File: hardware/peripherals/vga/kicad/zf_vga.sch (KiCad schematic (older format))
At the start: 3 parts

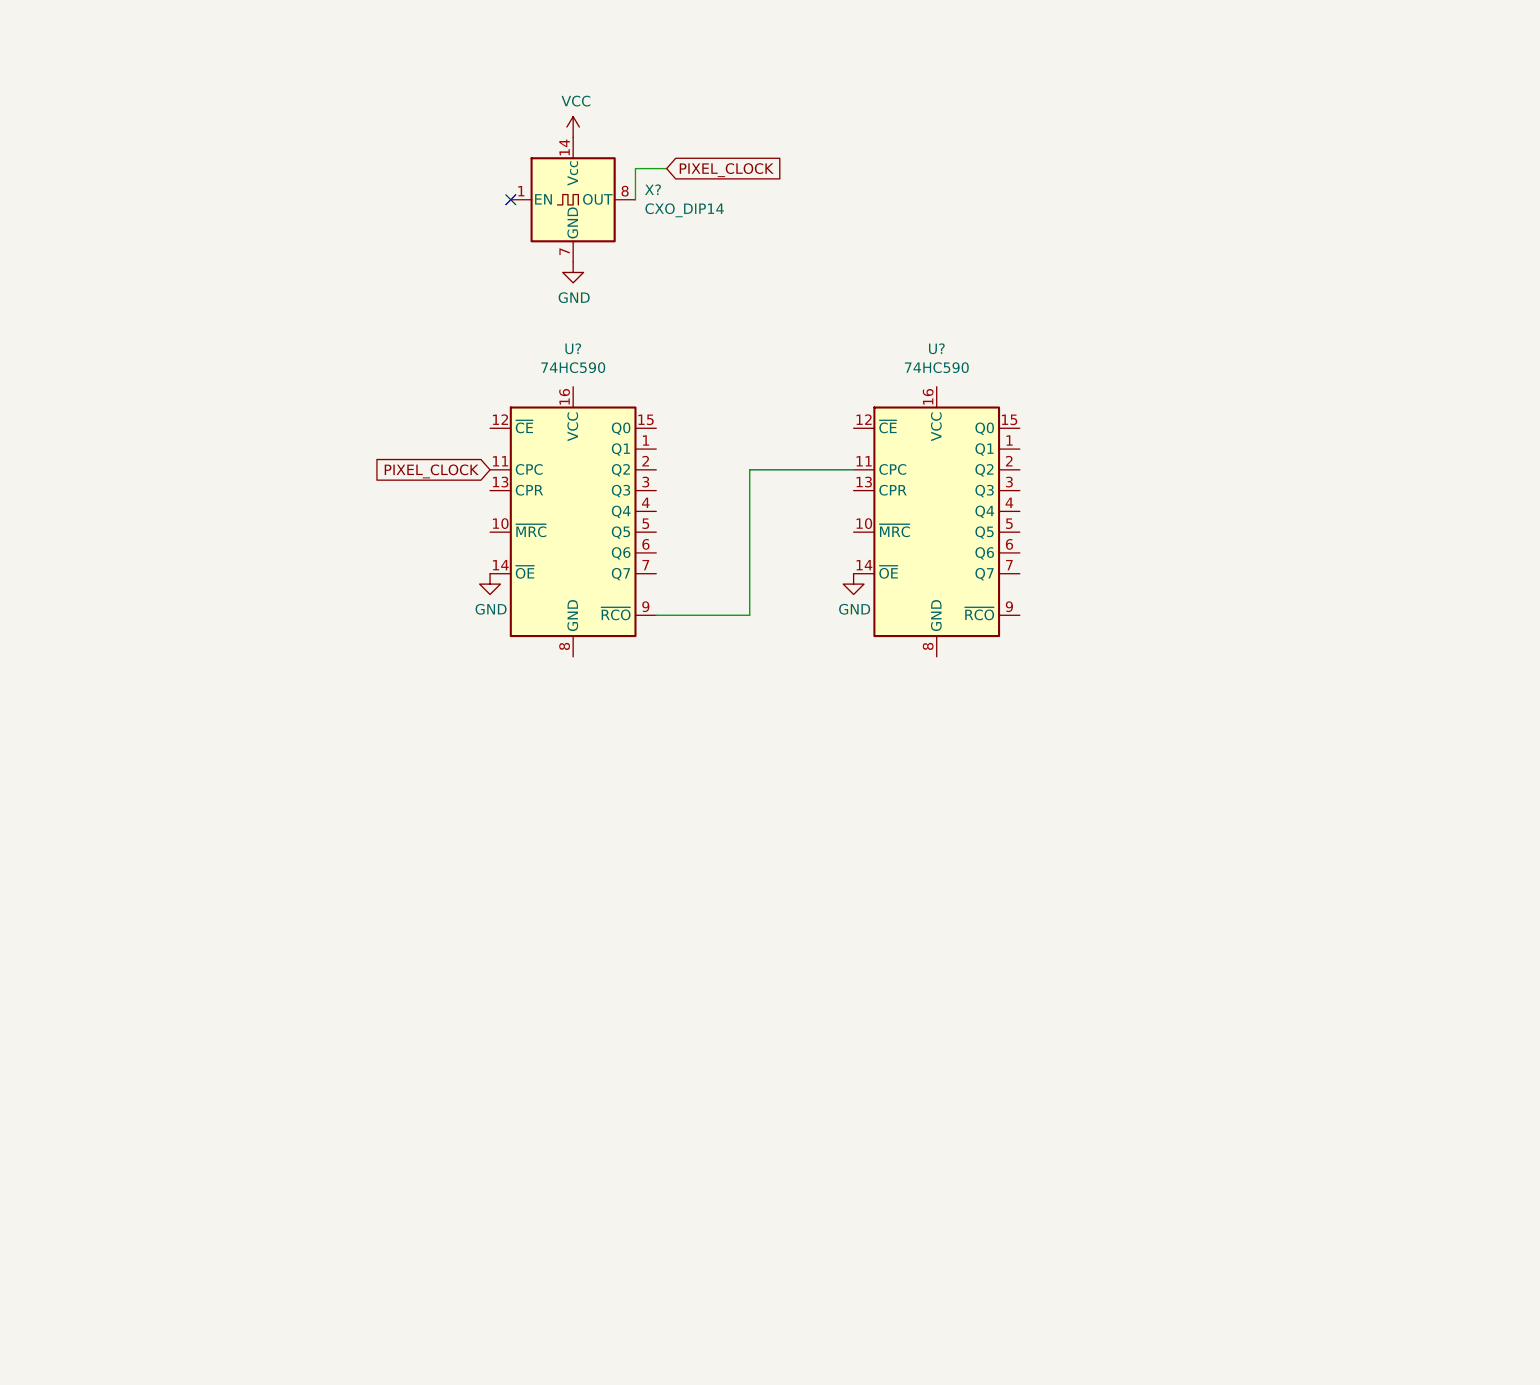
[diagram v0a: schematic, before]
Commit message: Generate test pattern
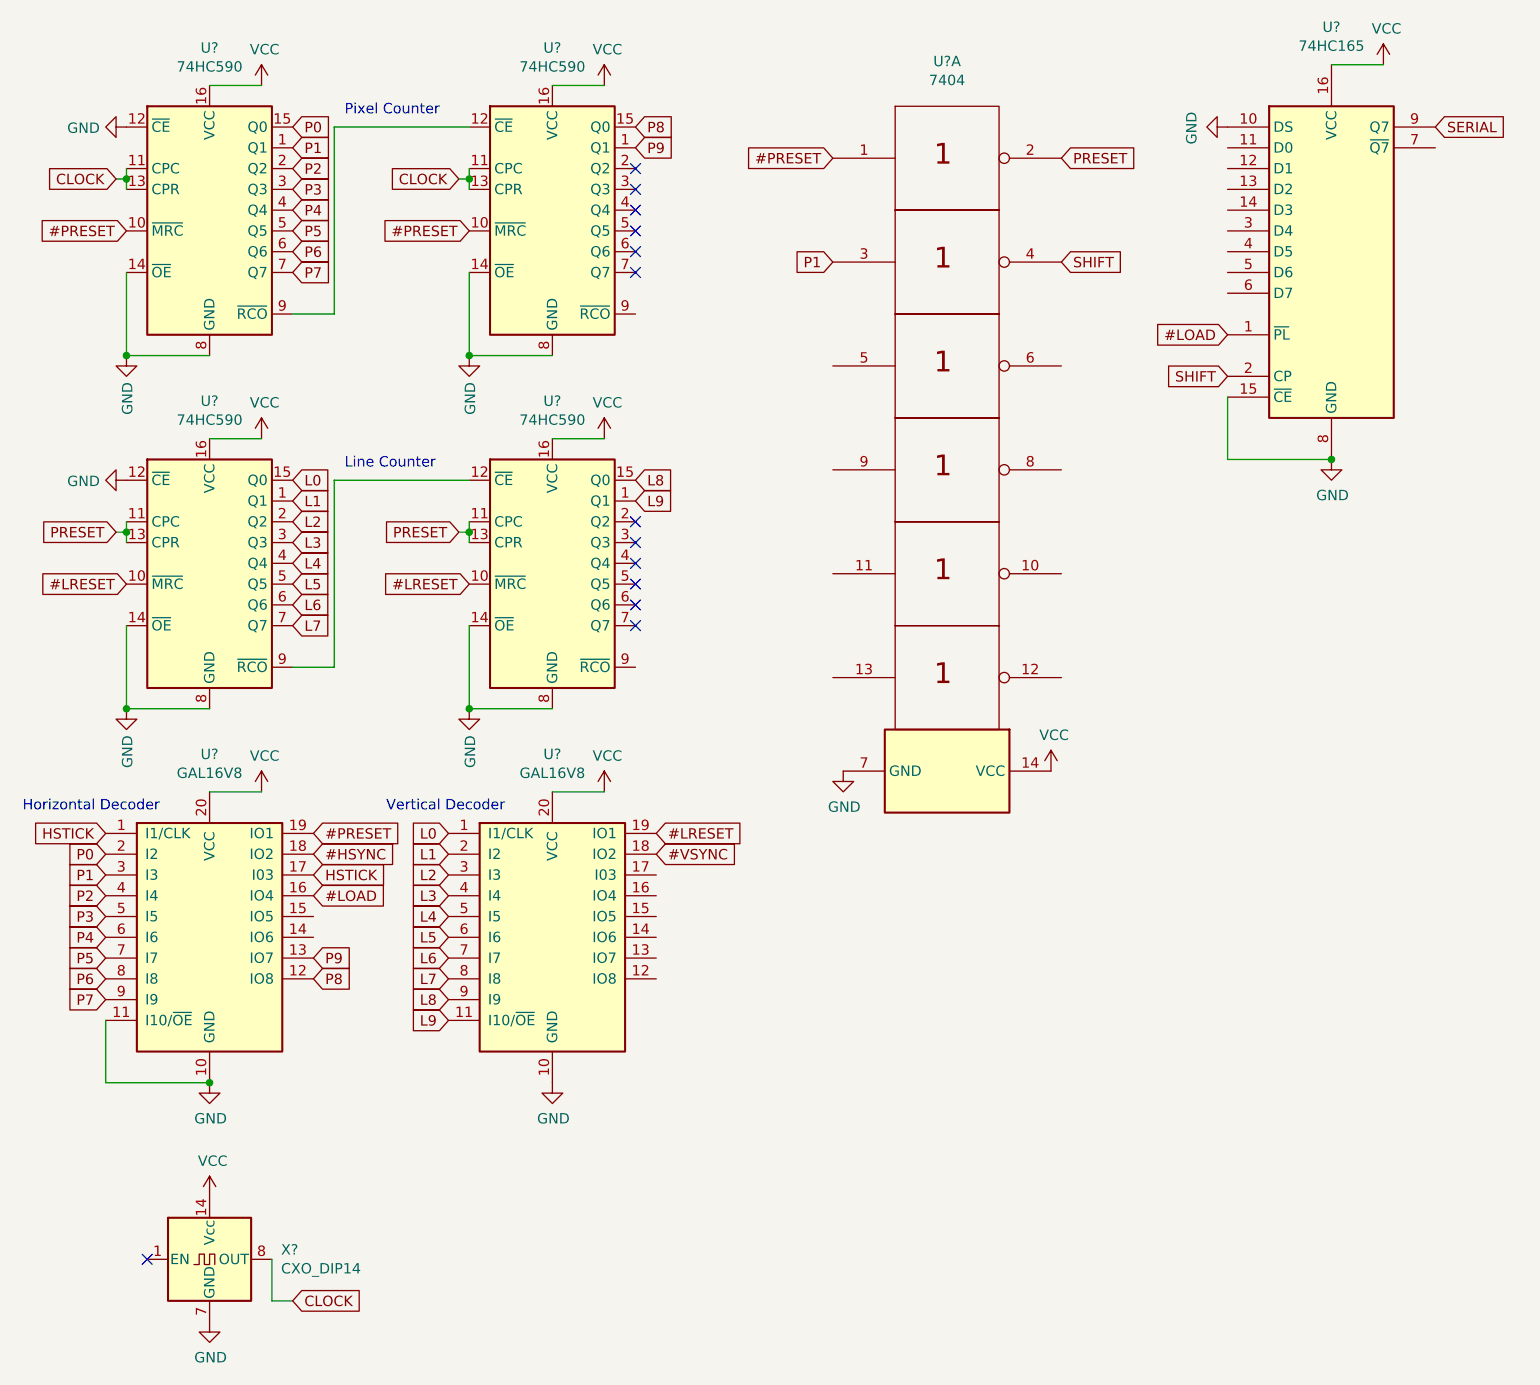
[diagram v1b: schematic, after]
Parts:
- removed U? (x2): 74HC590, symbol 74xx:74HC590
- added U? (x2): GAL16V8, symbol Logic_Programmable:GAL16V8
- added U? (x4): 74HC590, symbol 74xx:74HC590
- added U? (x6): 7404, symbol 74xx_IEEE:7404
- added U?: 74HC04, symbol 74xx:74HC04
- added U?: 74HC165, symbol 74xx:74HC165
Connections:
- net GND: now also U?.10 (DS), U?.10 (GND), U?.10 (GND), U?.11 (I10/~OE~), U?.12 (~CE), U?.12 (~CE), U?.14 (~OE), U?.14 (~OE), U?.14 (~OE), U?.14 (~OE), U?.15 (~CE), U?.7 (GND), U?.8 (GND), U?.8 (GND), U?.8 (GND), U?.8 (GND), U?.8 (GND)
- net VCC: now also U?.14 (VCC), U?.16 (VCC), U?.16 (VCC), U?.16 (VCC), U?.16 (VCC), U?.16 (VCC), U?.20 (VCC), U?.20 (VCC)
- net PIXEL_CLOCK renamed CLOCK
- net CLOCK: now also U?.11 (CPC), U?.11 (CPC), U?.13 (CPR), U?.13 (CPR)
- new net: U?.12 (~CE), U?.9 (~RCO) (x2)
- new net #HSYNC: U?.18 (IO2)
- new net #LOAD: U?.1 (~PL), U?.16 (IO4)
- new net #LRESET: U?.10 (~MRC), U?.10 (~MRC), U?.19 (IO1)
- new net #PRESET: U?.1, U?.10 (~MRC), U?.10 (~MRC), U?.19 (IO1)
- new net #VSYNC: U?.18 (IO2)
- new net Gnd: U?.14 (Vcc), U?.14 (Vcc), U?.14 (Vcc), U?.14 (Vcc), U?.14 (Vcc), U?.14 (Vcc), U?.7 (Gnd), U?.7 (Gnd), U?.7 (Gnd), U?.7 (Gnd), U?.7 (Gnd), U?.7 (Gnd)
- new net HSTICK: U?.1 (I1/CLK), U?.17 (I03)
- new net L0: U?.1 (I1/CLK), U?.15 (Q0)
- new net L1: U?.1 (Q1), U?.2 (I2)
- new net L2: U?.2 (Q2), U?.3 (I3)
- new net L3: U?.3 (Q3), U?.4 (I4)
- new net L4: U?.4 (Q4), U?.5 (I5)
- new net L5: U?.5 (Q5), U?.6 (I6)
- new net L6: U?.6 (Q6), U?.7 (I7)
- new net L7: U?.7 (Q7), U?.8 (I8)
- new net L8: U?.15 (Q0), U?.9 (I9)
- new net L9: U?.1 (Q1), U?.11 (I10/~OE~)
- new net P0: U?.15 (Q0), U?.2 (I2)
- new net P1: U?.1 (Q1), U?.3, U?.3 (I3)
- new net P2: U?.2 (Q2), U?.4 (I4)
- new net P3: U?.3 (Q3), U?.5 (I5)
- new net P4: U?.4 (Q4), U?.6 (I6)
- new net P5: U?.5 (Q5), U?.7 (I7)
- new net P6: U?.6 (Q6), U?.8 (I8)
- new net P7: U?.7 (Q7), U?.9 (I9)
- new net P8: U?.12 (IO8), U?.15 (Q0)
- new net P9: U?.1 (Q1), U?.13 (IO7)
- new net PRESET: U?.11 (CPC), U?.11 (CPC), U?.13 (CPR), U?.13 (CPR), U?.2
- new net SERIAL: U?.9 (Q7)
- new net SHIFT: U?.2 (CP), U?.4
- no-connect marks 1 -> 13
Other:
- note added: "Horizontal Decoder"
- note added: "Line Counter"
- note added: "Pixel Counter"
- note added: "Vertical Decoder"
- moved on the sheet: X?
